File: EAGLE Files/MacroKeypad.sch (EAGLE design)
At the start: 11 parts, among them IC1 ATMEGA32U4-AUR

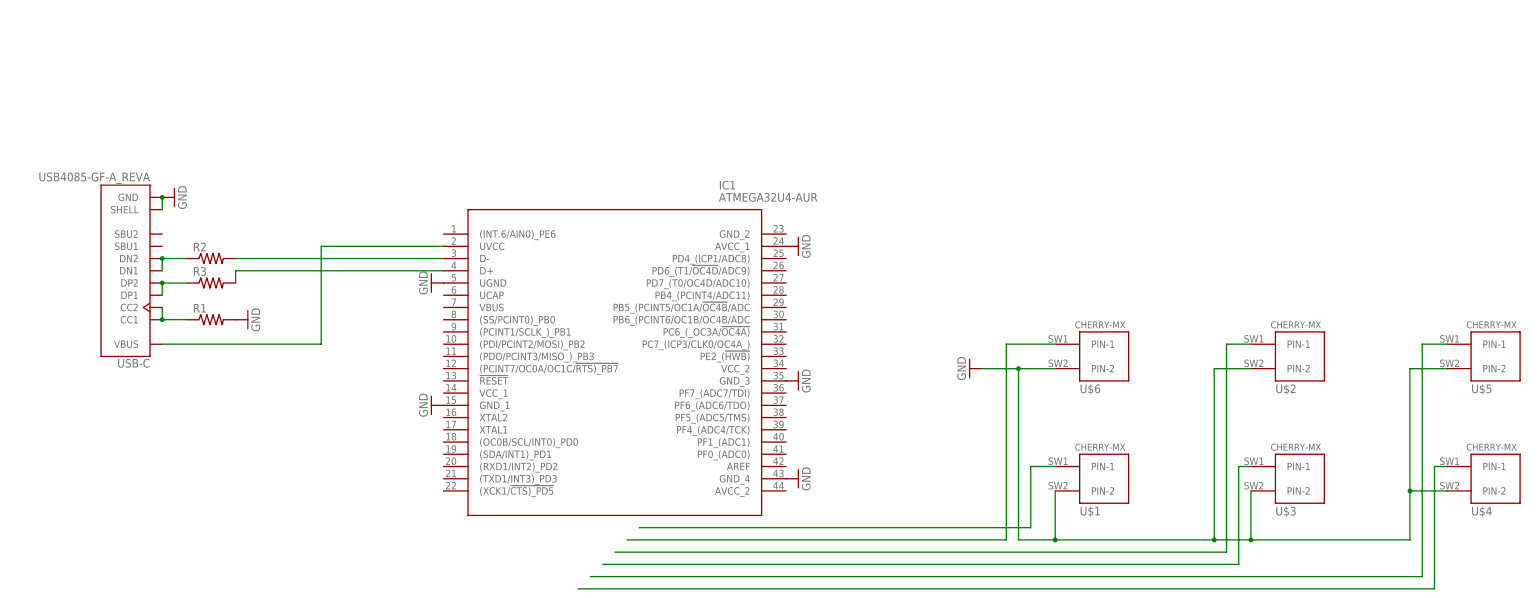
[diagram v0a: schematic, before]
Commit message: Update more files
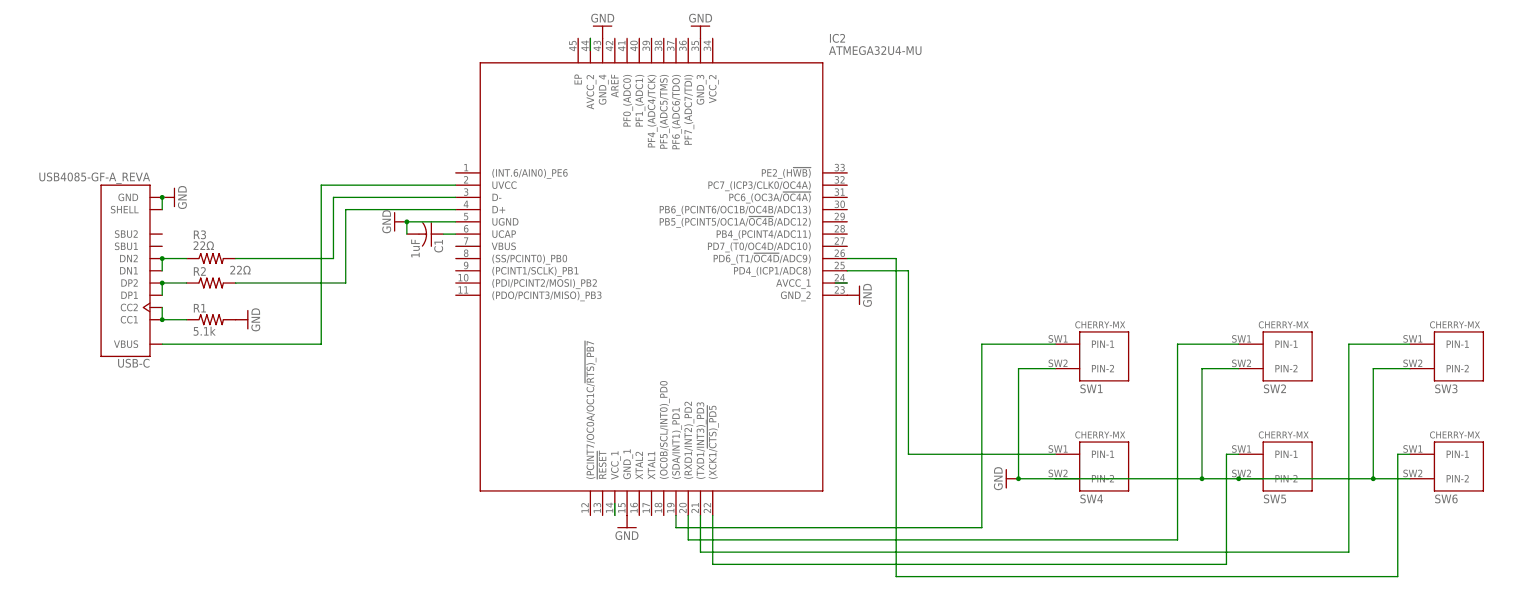
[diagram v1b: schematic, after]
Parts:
- removed IC1: ATMEGA32U4-AUR, SamacSys_Parts:ATMEGA32U4-AUR
- removed U$1, U$2, U$3, U$4, U$5: CHERRY-MX, cherrymx:CHERRY-MX
- added C1: 1uF, adafruit:C-USC0805
- added IC2: ATMEGA32U4-MU, SamacSys_Parts:ATMEGA32U4-MU
- added SW2, SW3, SW4, SW5, SW6: CHERRY-MX, cherrymx:CHERRY-MX
- R1: value (none) -> 5.1k
- R2, R3: value (none) -> 22Ω
- renumbered U$6 to SW1
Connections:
- net N$1 renamed CC
- removed net SW1: SW1.PIN-1
- removed net SW2: U$3.PIN-1
- removed net SW3: U$4.PIN-1
- removed net SW4: U$1.PIN-1
- removed net SW5: U$2.PIN-1
- removed net SW6: U$5.PIN-1
- new net D+: R2.1, USB-C.DP1, USB-C.DP2
- new net D+RES: IC2.D+, R2.2
- new net D-: R3.1, USB-C.DN1, USB-C.DN2
- new net D-RES: IC2.D-, R3.2
- new net N$1: IC2.(SDA/INT1)_PD1, SW1.PIN-1
- new net UCAP: C1.1, IC2.UCAP
- new net VCC: IC2.AVCC_1, IC2.AVCC_2, IC2.VCC_1
- new net VIN: IC2.UVCC, USB-C.VBUS
- net GND: now also C1.2, IC2.GND_1, IC2.GND_2, IC2.GND_3, IC2.GND_4, IC2.UGND, SW2.PIN-2, SW3.PIN-2, SW4.PIN-2, SW5.PIN-2, SW6.PIN-2; no longer IC1.AVCC_1, IC1.GND_1, IC1.GND_3, IC1.GND_4, IC1.UGND, U$1.PIN-2, U$2.PIN-2, U$3.PIN-2, U$4.PIN-2, U$5.PIN-2
- net N$2: now also IC2.(RXD1/INT2)_PD2, SW2.PIN-1; no longer IC1.UVCC, USB-C.VBUS
- net N$3: now also IC2.(TXD1/INT3)_PD3, SW3.PIN-1; no longer R3.1, USB-C.DP1, USB-C.DP2
- net N$4: now also IC2.PD4_(ICP1/ADC8), SW4.PIN-1; no longer R2.1, USB-C.DN1, USB-C.DN2
- net N$5: now also IC2.(XCK1/!CTS)_PD5, SW5.PIN-1; no longer IC1.D-, R2.2
- net N$6: now also IC2.PD6_(T1/!OC4D!/ADC9), SW6.PIN-1; no longer IC1.D+, R3.2
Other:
- moved on the sheet: R2, R3
